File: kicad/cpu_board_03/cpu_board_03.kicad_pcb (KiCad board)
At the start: 2 copper layers, 99.1 x 94.2 mm, 59 parts, among them J1 DIN41612_02x32_AC, J10 PLD_aux, J11 Conn_01x09, J6 Conn_01x02_Socket, J9 Ram1 Enable, SW1 SW_Reset, SW2 SW_PWR, U1 W65C02SxP, U10 74HC245, U11 74HC245, U12 74LS138, U13 74AHC1G32, U2 H3-65756H-5, U3 27C512, U4 ATF22V10, U5 74LS138, U6 74HCT574, U7 H3-65756H-5, U8 74HC245, U9 MAX1232, X1 ACO-14MHz

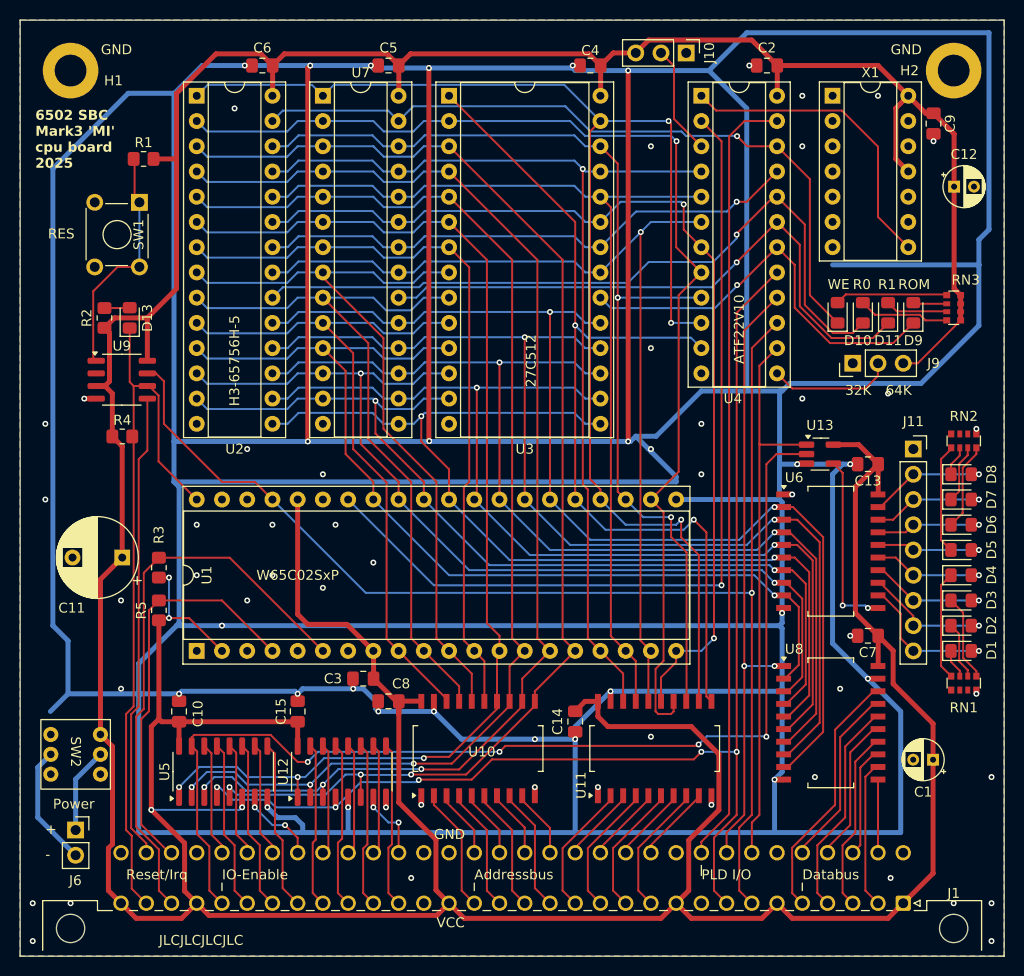
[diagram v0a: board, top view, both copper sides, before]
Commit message: cleaned up pullup mess
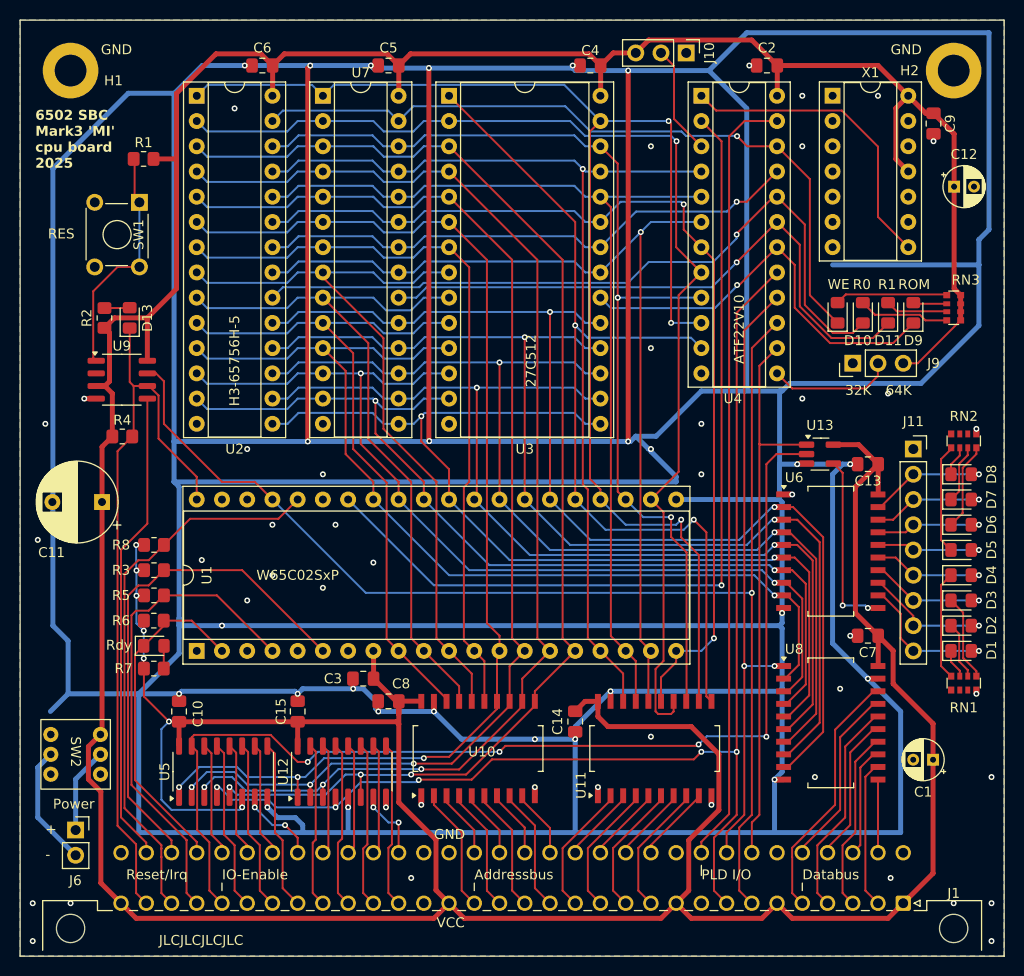
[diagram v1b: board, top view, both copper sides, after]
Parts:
- added D14: LED_Small, LED_SMD:LED_0805_2012Metric_Pad1.15x1.40mm_HandSolder, F.Cu at (46.5, 75.7)
- added R6: 10K, Resistor_SMD:R_0805_2012Metric_Pad1.20x1.40mm_HandSolder, F.Cu at (46.5, 73.2)
- added R7: 10K, Resistor_SMD:R_0805_2012Metric_Pad1.20x1.40mm_HandSolder, F.Cu at (46.5, 78.0)
- added R8: 10K, Resistor_SMD:R_0805_2012Metric_Pad1.20x1.40mm_HandSolder, F.Cu at (46.5, 65.5)
- moved C11 5.95 mm to (41.3, 61.2)
- moved R5 1.59 mm to (46.5, 70.6), turned to 0 degrees
- moved R3 0.55 mm to (46.5, 68.1), turned to 0 degrees
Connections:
- J1 pad a29: VCC -> /~{IRQ}
- J1 pad a30: /~{NMI} -> /BE
- J1 pad c29: GND -> /RDY
- J1 pad c30: /~{IRQ} -> /~{NMI}
- U1 pad 2: VCC -> /RDY
- U1 pad 36: VCC -> /BE
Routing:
- net /BE: track 0.00 -> 55.6 mm
- net /RDY: track 0.00 -> 34.3 mm
- net VCC: track 538.4 -> 512.2 mm, vias 4 -> 7
- net /~{IRQ}: track 41.1 -> 49.1 mm
- net /~{NMI}: track 57.6 -> 51.7 mm
- net Net-(D14-A): track 0.00 -> 2.30 mm
- net /RES: track 47.0 -> 47.9 mm
- net /~{RES}: track 74.3 -> 74.9 mm
- net GND: track 928.8 -> 928.2 mm, vias 74 -> 71
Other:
- board text added: "Rdy"
